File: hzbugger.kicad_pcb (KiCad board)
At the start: 2 copper layers, 55.4 x 26.7 mm, 54 parts, among them J2 IDC, J4 SWD, J6 GPIO, SW1 RESET_SW, SW2 BOOT0_SW, U1 STM32F103C8T6, U2 SRV05-4, U3 AMS1117-3.3, U4 HX AM 90D, Y1 8M

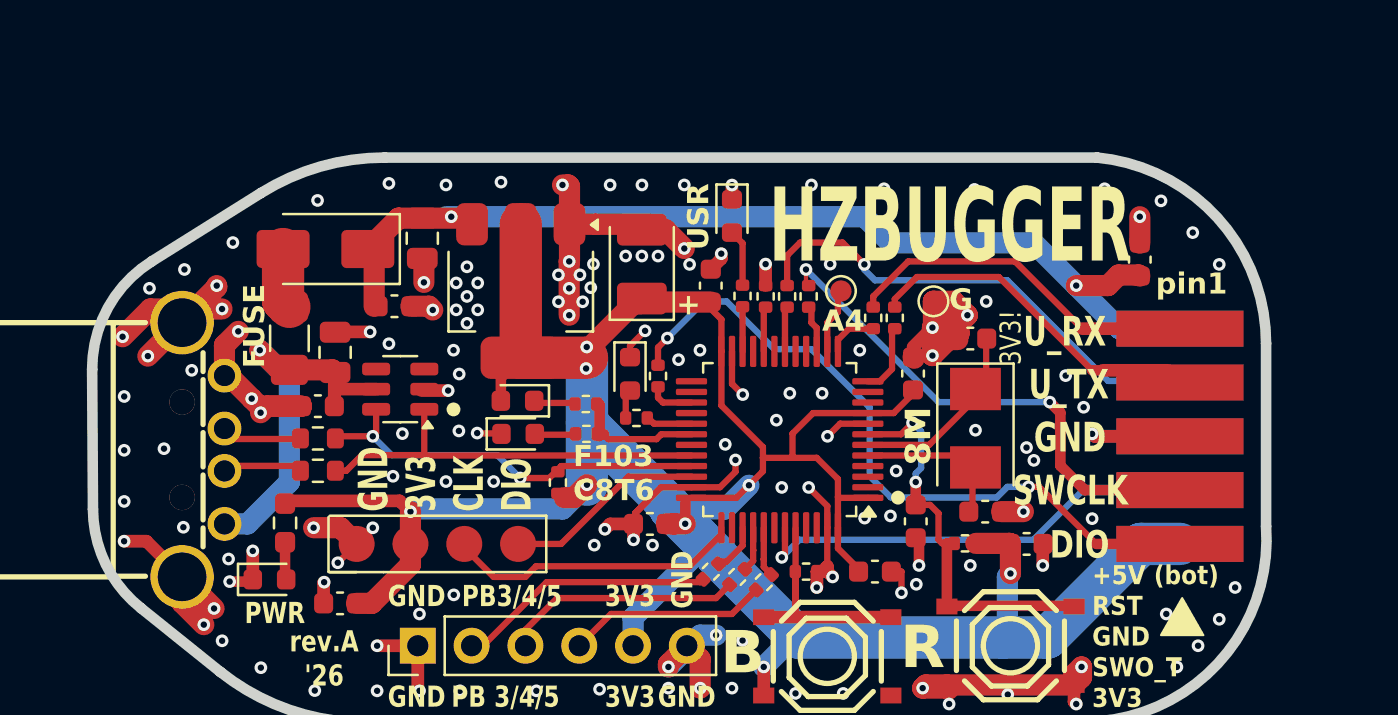
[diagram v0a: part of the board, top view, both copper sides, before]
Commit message: layout enhancements
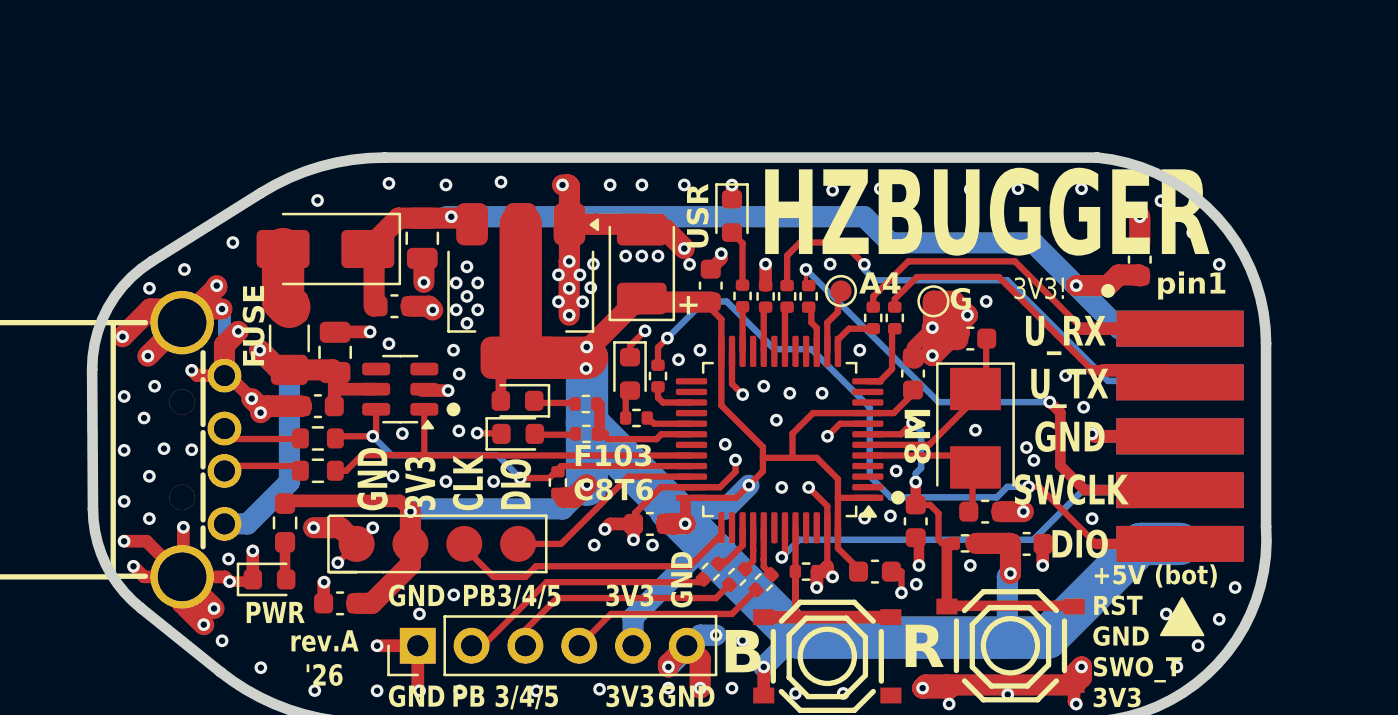
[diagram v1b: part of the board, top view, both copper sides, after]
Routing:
- net GND: track 127.3 -> 140.0 mm, vias 148 -> 156
